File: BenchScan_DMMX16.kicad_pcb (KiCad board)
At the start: 4 copper layers, 220 x 110 mm, 113 parts, among them J1 Phoenix 1190370 8POS, J10 POMONA 73099 BLACK, J11 POMONA 73099 RED, J12 POMONA 73099 BLACK, J2 Phoenix 1190370 8POS, J3 Phoenix 1190370 8POS, J4 Phoenix 1190370 8POS, J5 691137710006 DMM, J6 POMONA 73099 RED, J7 54-00129 BARREL 5V, J8 POMONA 73099 BLACK, J9 POMONA 73099 RED, K1 UD2-5NE, K10 UD2-5NE, K11 UD2-5NE, K12 UD2-5NE, K13 UD2-5NE, K14 UD2-5NE, K15 UD2-5NE, K16 UD2-5NE, K17 UD2-5NE, K2 UD2-5NE, K3 UD2-5NE, K4 UD2-5NE, K5 UD2-5NE, K6 UD2-5NE, K7 UD2-5NE, K8 UD2-5NE, K9 UD2-5NE, Q1 2N7002K, Q10 2N7002K, Q11 2N7002K, Q12 2N7002K, Q13 2N7002K, Q14 2N7002K, Q15 2N7002K, Q16 2N7002K, Q17 2N7002K, Q19 AO3401A, Q2 2N7002K, Q3 2N7002K, Q4 2N7002K, Q5 2N7002K, Q6 2N7002K, Q7 2N7002K, Q8 2N7002K, Q9 2N7002K, U1 XIAO ESP32-C6 / 113991254, U2 SN74HC595PWR, U3 SN74HC595PWR

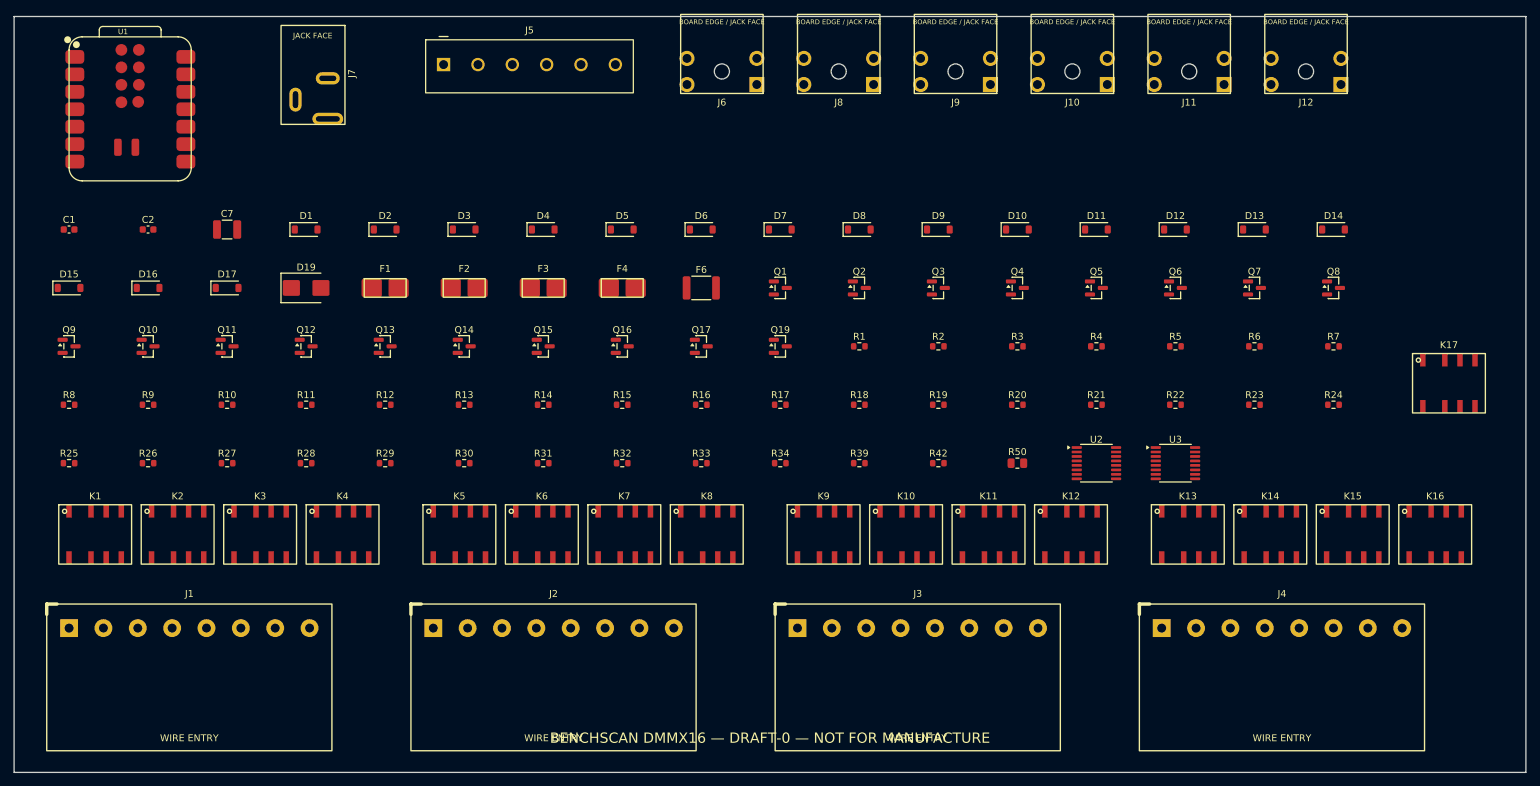
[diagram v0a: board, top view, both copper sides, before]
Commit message: Optimize relay driver placement
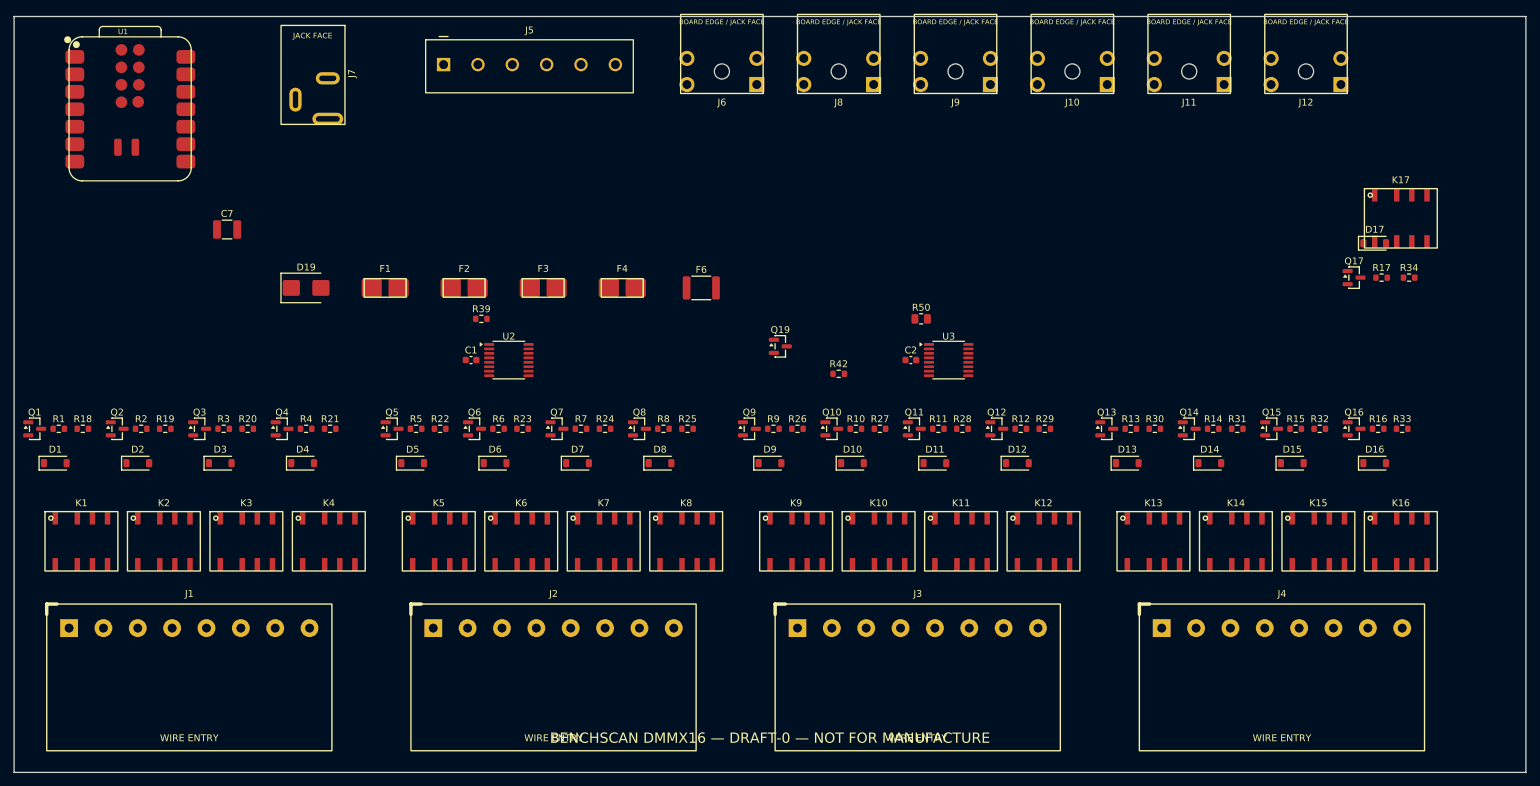
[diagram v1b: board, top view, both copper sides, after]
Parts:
- moved D16 180.3 mm to (238.0, 97.0)
- moved D15 179.8 mm to (226.0, 97.0)
- moved D17 167.1 mm to (238.0, 65.0)
- moved R1 117.1 mm to (46.5, 92.0)
- moved R2 116.6 mm to (58.5, 92.0)
- moved R3 116.1 mm to (70.5, 92.0)
- moved R4 115.6 mm to (82.5, 92.0)
- moved R18 113.1 mm to (50.0, 92.0)
- moved C2 112.6 mm to (170.5, 82.0)
- moved R19 112.6 mm to (62.0, 92.0)
- moved R20 112.1 mm to (74.0, 92.0)
- moved R21 111.6 mm to (86.0, 92.0)
- moved R5 111.1 mm to (98.5, 92.0)
- moved R6 110.7 mm to (110.5, 92.0)
- moved Q1 110.4 mm to (43.0, 92.0)
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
